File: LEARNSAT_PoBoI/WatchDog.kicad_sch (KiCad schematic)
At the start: 12 parts, among them SW801 B3U-1000P, SW802 B3U-1000P, U801 MAX6746KA29+T, U802 MAX6746KA29+T, U803 SN74AUP1G08QDCKRQ1, U804 SN74AUP1G08QDCKRQ1

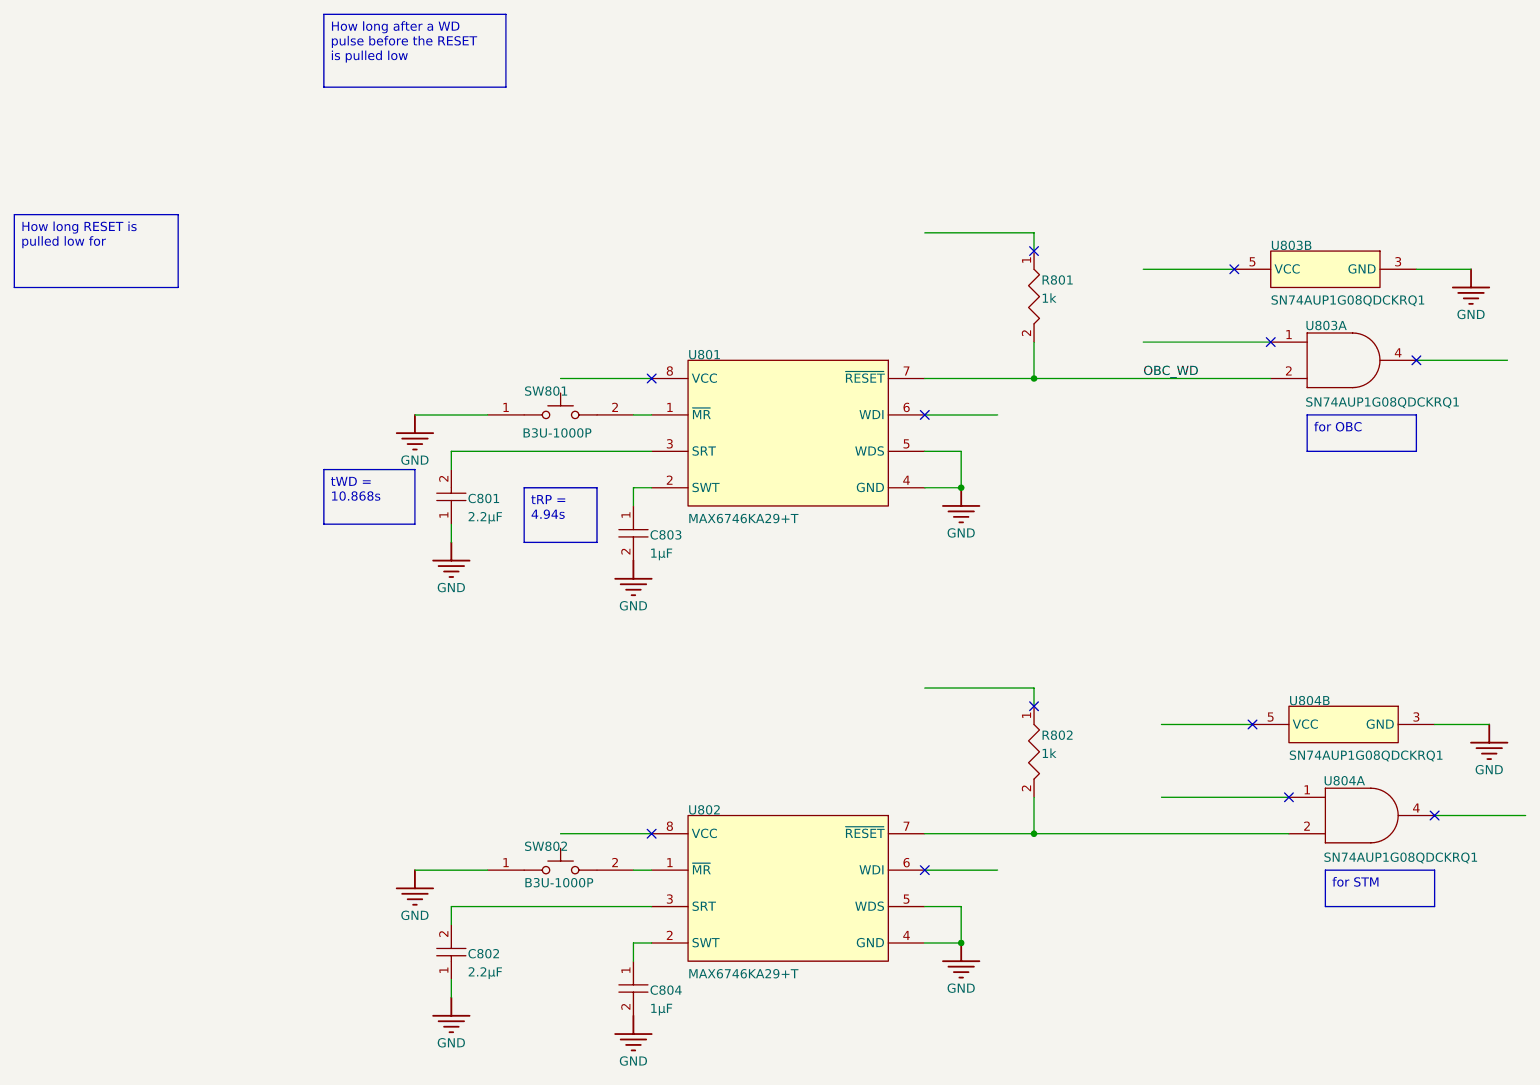
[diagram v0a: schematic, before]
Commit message: Add files via upload
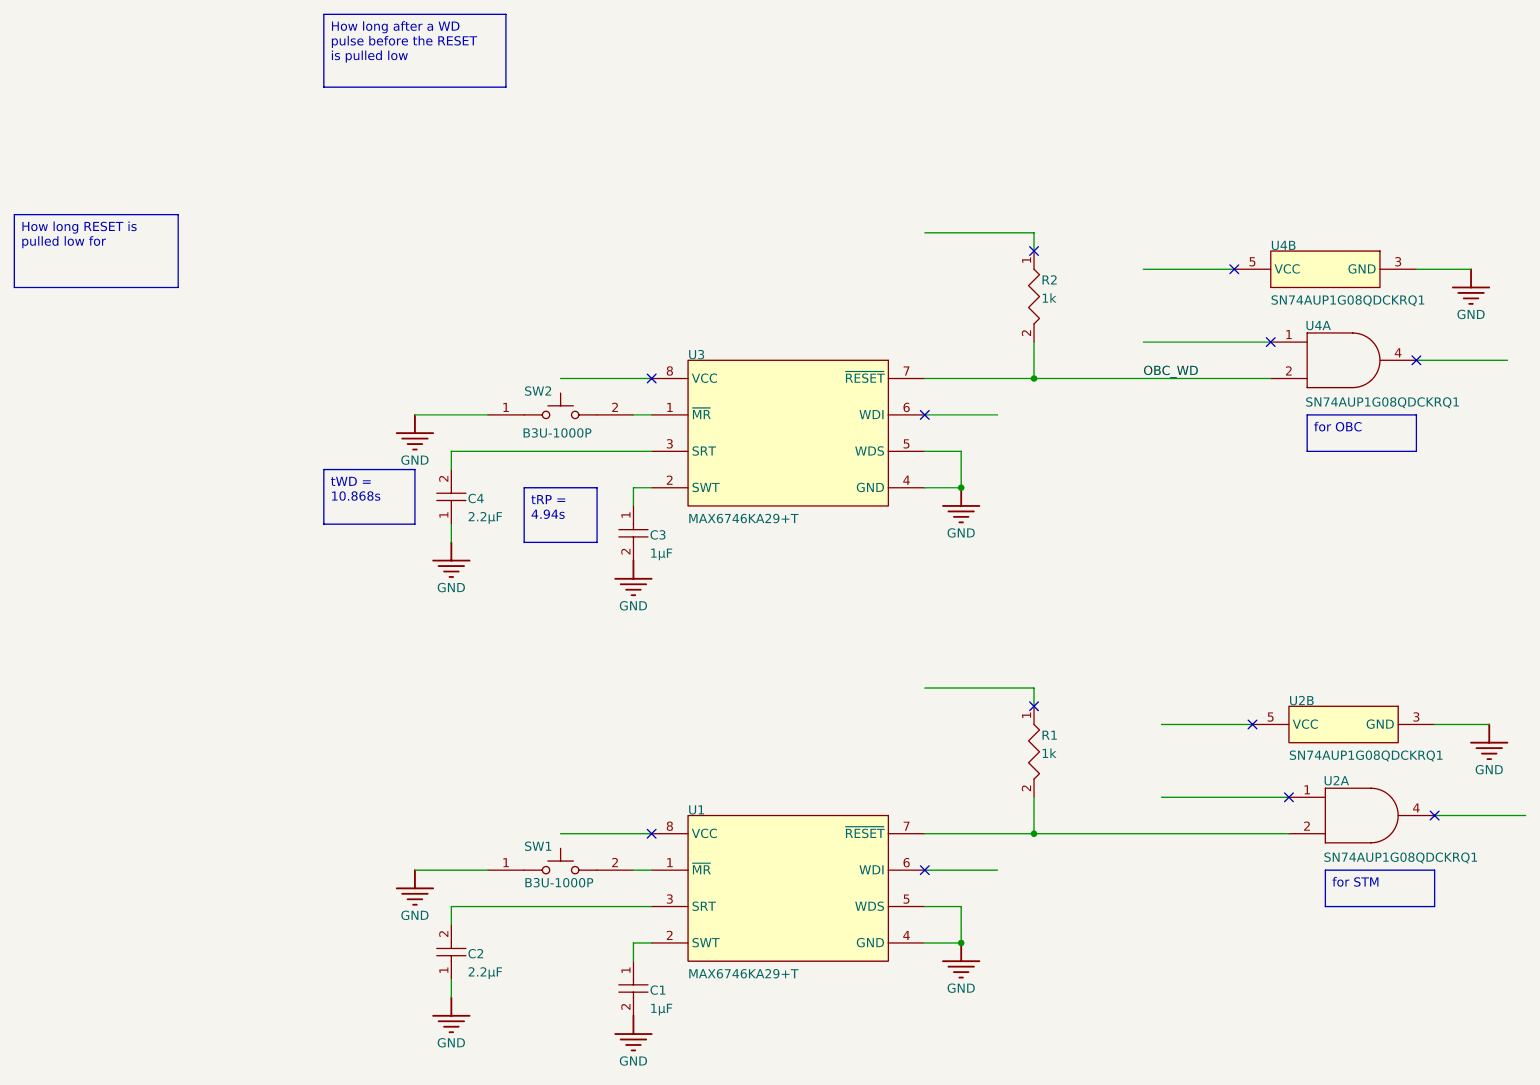
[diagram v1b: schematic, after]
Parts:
- C1: renamed from C804; footprint Capacitor_SMD:C_0603_1608Metric -> CAPC0603(1608)100_L
- C2: renamed from C802; footprint Capacitor_SMD:C_0402_1005Metric -> CAPC0402(1005)60_L
- C3: renamed from C803; footprint Capacitor_SMD:C_0603_1608Metric -> CAPC0603(1608)100_L
- C4: renamed from C801; footprint Capacitor_SMD:C_0402_1005Metric -> CAPC0402(1005)60_L
- R1: renamed from R802; footprint Resistor_SMD:R_0805_2012Metric -> RESC0805(2012)_L
- R2: renamed from R801; footprint Resistor_SMD:R_0805_2012Metric -> RESC0805(2012)_L
- SW1: renamed from SW802; footprint B3U-1000P:SW_B3U-1000P -> OMRON-B3U-1000_V
- SW2: renamed from SW801; footprint B3U-1000P:SW_B3U-1000P -> OMRON-B3U-1000_V
- U1: renamed from U802; footprint MAX6746KA29_T:SOT65P280X145-8N -> FP-K8-5-IPC_C
- U2: renamed from U804; footprint SN74AUP1G08QDCKRQ1:SOT65P210X110-5N -> DCK0005A_N
- U3: renamed from U801; footprint MAX6746KA29_T:SOT65P280X145-8N -> FP-K8-5-IPC_C
- U4: renamed from U803; footprint SN74AUP1G08QDCKRQ1:SOT65P210X110-5N -> DCK0005A_N
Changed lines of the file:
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@@
 		(on_board yes)
 		(dnp no)
-		(property "Reference" "#PWR0806"
+		(property "Reference" "#PWR?"
 			(at 96.52 172.72 0)
 			(effects
@@
 			(project ""
 				(path "/31302da5-a970-4b2b-aa05-afcd06cb9d09/24205a11-7394-4676-a8e1-3f02d7a9d0eb"
-					(reference "#PWR0806")
+					(reference "#PWR?")
 					(unit 1)
 				)
@@
 		(on_board yes)
 		(dnp no)
-		(property "Reference" "R802"
+		(property "Reference" "R1"
 			(at 153.416 134.366 0)
 			(effects
@@
 			)
 		)
-		(property "Footprint" "Resistor_SMD:R_0805_2012Metric"
+		(property "Footprint" "RESC0805(2012)_L"
 			(at 152.4 129.54 0)
 			(effects
@@
 			(project ""
 				(path "/31302da5-a970-4b2b-aa05-afcd06cb9d09/24205a11-7394-4676-a8e1-3f02d7a9d0eb"
-					(reference "R802")
+					(reference "R1")
 					(unit 1)
 				)
@@
 		(on_board yes)
 		(dnp no)
-		(property "Reference" "C803"
+		(property "Reference" "C3"
 			(at 98.806 106.426 0)
 			(effects
@@
 			)
 		)
-		(property "Footprint" "Capacitor_SMD:C_0603_1608Metric"
+		(property "Footprint" "CAPC0603(1608)100_L"
 			(at 96.52 101.6 0)
 			(effects
@@
 			(project ""
 				(path "/31302da5-a970-4b2b-aa05-afcd06cb9d09/24205a11-7394-4676-a8e1-3f02d7a9d0eb"
-					(reference "C803")
+					(reference "C3")
 					(unit 1)
 				)
@@
 		(on_board yes)
 		(dnp no)
-		(property "Reference" "#PWR0807"
+		(property "Reference" "#PWR?"
 			(at 142.24 99.06 0)
 			(effects
@@
 			(project ""
 				(path "/31302da5-a970-4b2b-aa05-afcd06cb9d09/24205a11-7394-4676-a8e1-3f02d7a9d0eb"
-					(reference "#PWR0807")
+					(reference "#PWR?")
 					(unit 1)
 				)
@@
 		(on_board yes)
 		(dnp no)
-		(property "Reference" "C804"
+		(property "Reference" "C1"
 			(at 98.806 169.926 0)
 			(effects
@@
 			)
 		)
-		(property "Footprint" "Capacitor_SMD:C_0603_1608Metric"
+		(property "Footprint" "CAPC0603(1608)100_L"
 			(at 96.52 165.1 0)
 			(effects
@@
 			(project ""
 				(path "/31302da5-a970-4b2b-aa05-afcd06cb9d09/24205a11-7394-4676-a8e1-3f02d7a9d0eb"
-					(reference "C804")
+					(reference "C1")
 					(unit 1)
 				)
@@
 		(on_board yes)
 		(dnp no)
-		(property "Reference" "R801"
+		(property "Reference" "R2"
 			(at 153.416 70.866 0)
 			(effects
@@
 			)
 		)
-		(property "Footprint" "Resistor_SMD:R_0805_2012Metric"
+		(property "Footprint" "RESC0805(2012)_L"
 			(at 152.4 66.04 0)
 			(effects
@@
 			(project ""
 				(path "/31302da5-a970-4b2b-aa05-afcd06cb9d09/24205a11-7394-4676-a8e1-3f02d7a9d0eb"
-					(reference "R801")
+					(reference "R2")
 					(unit 1)
 				)
@@
 		(on_board yes)
 		(dnp no)
-		(property "Reference" "C802"
+		(property "Reference" "C2"
 			(at 73.406 164.846 0)
 			(effects
@@
 			)
 		)
-		(property "Footprint" "Capacitor_SMD:C_0402_1005Metric"
+		(property "Footprint" "CAPC0402(1005)60_L"
 			(at 71.12 167.64 0)
 			(effects
@@
 			(project ""
 				(path "/31302da5-a970-4b2b-aa05-afcd06cb9d09/24205a11-7394-4676-a8e1-3f02d7a9d0eb"
-					(reference "C802")
+					(reference "C2")
 					(unit 1)
 				)
@@
 		(on_board yes)
 		(dnp no)
-		(property "Reference" "#PWR0804"
+		(property "Reference" "#PWR?"
 			(at 71.12 170.18 0)
 			(effects
@@
 			(project ""
 				(path "/31302da5-a970-4b2b-aa05-afcd06cb9d09/24205a11-7394-4676-a8e1-3f02d7a9d0eb"
-					(reference "#PWR0804")
+					(reference "#PWR?")
 					(unit 1)
 				)
@@
 		(on_board yes)
 		(dnp no)
-		(property "Reference" "#PWR0802"
+		(property "Reference" "#PWR?"
 			(at 66.04 152.4 0)
 			(effects
@@
 			(project ""
 				(path "/31302da5-a970-4b2b-aa05-afcd06cb9d09/24205a11-7394-4676-a8e1-3f02d7a9d0eb"
-					(reference "#PWR0802")
+					(reference "#PWR?")
 					(unit 1)
 				)
@@
 		(on_board yes)
 		(dnp no)
-		(property "Reference" "U801"
+		(property "Reference" "U3"
 			(at 104.14 81.28 0)
 			(effects
@@
 			)
 		)
-		(property "Footprint" "MAX6746KA29_T:SOT65P280X145-8N"
+		(property "Footprint" "FP-K8-5-IPC_C"
 			(at 99.06 83.82 0)
 			(effects
@@
 			(project ""
 				(path "/31302da5-a970-4b2b-aa05-afcd06cb9d09/24205a11-7394-4676-a8e1-3f02d7a9d0eb"
-					(reference "U801")
+					(reference "U3")
 					(unit 1)
 				)
@@
 		(on_board yes)
 		(dnp no)
-		(property "Reference" "#PWR0803"
+		(property "Reference" "#PWR?"
 			(at 71.12 106.68 0)
 			(effects
@@
 			(project ""
 				(path "/31302da5-a970-4b2b-aa05-afcd06cb9d09/24205a11-7394-4676-a8e1-3f02d7a9d0eb"
-					(reference "#PWR0803")
+					(reference "#PWR?")
 					(unit 1)
 				)
@@
 		(on_board yes)
 		(dnp no)
-		(property "Reference" "U803"
+		(property "Reference" "U4"
 			(at 185.42 66.04 0)
 			(effects
@@
 			)
 		)
-		(property "Footprint" "SN74AUP1G08QDCKRQ1:SOT65P210X110-5N"
+		(property "Footprint" "DCK0005A_N"
 			(at 185.42 66.04 0)
 			(effects
@@
 			(project ""
 				(path "/31302da5-a970-4b2b-aa05-afcd06cb9d09/24205a11-7394-4676-a8e1-3f02d7a9d0eb"
-					(reference "U803")
+					(reference "U4")
 					(unit 2)
 				)
@@
 		(on_board yes)
 		(dnp no)
-		(property "Reference" "C801"
+		(property "Reference" "C4"
 			(at 73.406 101.346 0)
 			(effects
@@
 			)
 		)
-		(property "Footprint" "Capacitor_SMD:C_0402_1005Metric"
+		(property "Footprint" "CAPC0402(1005)60_L"
 			(at 71.12 104.14 0)
 			(effects
@@
 			(project ""
 				(path "/31302da5-a970-4b2b-aa05-afcd06cb9d09/24205a11-7394-4676-a8e1-3f02d7a9d0eb"
-					(reference "C801")
+					(reference "C4")
 					(unit 1)
 				)
@@
 		(on_board yes)
 		(dnp no)
-		(property "Reference" "#PWR0810"
+		(property "Reference" "#PWR?"
 			(at 215.9 132.08 0)
 			(effects
@@
 			(project ""
 				(path "/31302da5-a970-4b2b-aa05-afcd06cb9d09/24205a11-7394-4676-a8e1-3f02d7a9d0eb"
-					(reference "#PWR0810")
+					(reference "#PWR?")
 					(unit 1)
 				)
@@
 		(on_board yes)
 		(dnp no)
-		(property "Reference" "SW801"
+		(property "Reference" "SW2"
 			(at 81.28 86.36 0)
 			(effects
@@
 			)
 		)
-		(property "Footprint" "B3U-1000P:SW_B3U-1000P"
+		(property "Footprint" "OMRON-B3U-1000_V"
 			(at 81.28 86.36 0)
 			(effects
@@
 			(project ""
 				(path "/31302da5-a970-4b2b-aa05-afcd06cb9d09/24205a11-7394-4676-a8e1-3f02d7a9d0eb"
-					(reference "SW801")
+					(reference "SW2")
 					(unit 1)
 				)
@@
 		(on_board yes)
 		(dnp no)
-		(property "Reference" "#PWR0808"
+		(property "Reference" "#PWR?"
 			(at 142.24 162.56 0)
 			(effects
@@
 			(project ""
 				(path "/31302da5-a970-4b2b-aa05-afcd06cb9d09/24205a11-7394-4676-a8e1-3f02d7a9d0eb"
-					(reference "#PWR0808")
+					(reference "#PWR?")
 					(unit 1)
 				)
@@
 		(on_board yes)
 		(dnp no)
-		(property "Reference" "#PWR0805"
+		(property "Reference" "#PWR?"
 			(at 96.52 109.22 0)
 			(effects
@@
 			(project ""
 				(path "/31302da5-a970-4b2b-aa05-afcd06cb9d09/24205a11-7394-4676-a8e1-3f02d7a9d0eb"
-					(reference "#PWR0805")
+					(reference "#PWR?")
 					(unit 1)
 				)
@@
 		(on_board yes)
 		(dnp no)
-		(property "Reference" "#PWR0809"
+		(property "Reference" "#PWR?"
 			(at 213.36 68.58 0)
 			(effects
@@
 			(project ""
 				(path "/31302da5-a970-4b2b-aa05-afcd06cb9d09/24205a11-7394-4676-a8e1-3f02d7a9d0eb"
-					(reference "#PWR0809")
+					(reference "#PWR?")
 					(unit 1)
 				)
@@
 		(on_board yes)
 		(dnp no)
-		(property "Reference" "U804"
+		(property "Reference" "U2"
 			(at 192.786 140.716 0)
 			(effects
@@
 			)
 		)
-		(property "Footprint" "SN74AUP1G08QDCKRQ1:SOT65P210X110-5N"
+		(property "Footprint" "DCK0005A_N"
 			(at 193.04 139.7 0)
 			(effects
@@
 			(project ""
 				(path "/31302da5-a970-4b2b-aa05-afcd06cb9d09/24205a11-7394-4676-a8e1-3f02d7a9d0eb"
-					(reference "U804")
+					(reference "U2")
 					(unit 1)
 				)
@@
 		(on_board yes)
 		(dnp no)
-		(property "Reference" "#PWR0801"
+		(property "Reference" "#PWR?"
 			(at 66.04 88.9 0)
 			(effects
@@
 			(project ""
 				(path "/31302da5-a970-4b2b-aa05-afcd06cb9d09/24205a11-7394-4676-a8e1-3f02d7a9d0eb"
-					(reference "#PWR0801")
+					(reference "#PWR?")
 					(unit 1)
 				)
@@
 		(on_board yes)
 		(dnp no)
-		(property "Reference" "U803"
+		(property "Reference" "U4"
 			(at 190.246 77.216 0)
 			(effects
@@
 			)
 		)
-		(property "Footprint" "SN74AUP1G08QDCKRQ1:SOT65P210X110-5N"
+		(property "Footprint" "DCK0005A_N"
 			(at 190.5 76.2 0)
 			(effects
@@
 			(project ""
 				(path "/31302da5-a970-4b2b-aa05-afcd06cb9d09/24205a11-7394-4676-a8e1-3f02d7a9d0eb"
-					(reference "U803")
+					(reference "U4")
 					(unit 1)
 				)
@@
 		(on_board yes)
 		(dnp no)
-		(property "Reference" "U804"
+		(property "Reference" "U2"
 			(at 187.96 129.54 0)
 			(effects
@@
 			)
 		)
-		(property "Footprint" "SN74AUP1G08QDCKRQ1:SOT65P210X110-5N"
+		(property "Footprint" "DCK0005A_N"
 			(at 187.96 129.54 0)
 			(effects
@@
 			(project ""
 				(path "/31302da5-a970-4b2b-aa05-afcd06cb9d09/24205a11-7394-4676-a8e1-3f02d7a9d0eb"
-					(reference "U804")
+					(reference "U2")
 					(unit 2)
 				)
@@
 		(on_board yes)
 		(dnp no)
-		(property "Reference" "SW802"
+		(property "Reference" "SW1"
 			(at 81.28 149.86 0)
 			(effects
@@
 			)
 		)
-		(property "Footprint" "B3U-1000P:SW_B3U-1000P"
+		(property "Footprint" "OMRON-B3U-1000_V"
 			(at 81.28 149.86 0)
 			(effects
@@
 			(project ""
 				(path "/31302da5-a970-4b2b-aa05-afcd06cb9d09/24205a11-7394-4676-a8e1-3f02d7a9d0eb"
-					(reference "SW802")
+					(reference "SW1")
 					(unit 1)
 				)
@@
 		(on_board yes)
 		(dnp no)
-		(property "Reference" "U802"
+		(property "Reference" "U1"
 			(at 104.14 144.78 0)
 			(effects
@@
 			)
 		)
-		(property "Footprint" "MAX6746KA29_T:SOT65P280X145-8N"
+		(property "Footprint" "FP-K8-5-IPC_C"
 			(at 99.06 147.32 0)
 			(effects
@@
 			(project ""
 				(path "/31302da5-a970-4b2b-aa05-afcd06cb9d09/24205a11-7394-4676-a8e1-3f02d7a9d0eb"
-					(reference "U802")
+					(reference "U1")
 					(unit 1)
 				)
